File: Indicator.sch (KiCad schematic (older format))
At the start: 6 parts, among them U10 BC56-12SURKWA, U11 SC56-11SRWA, U12 MAX7219EWG+T, U8 CC56-12SURKWA, U9 MAX7219EWG+T

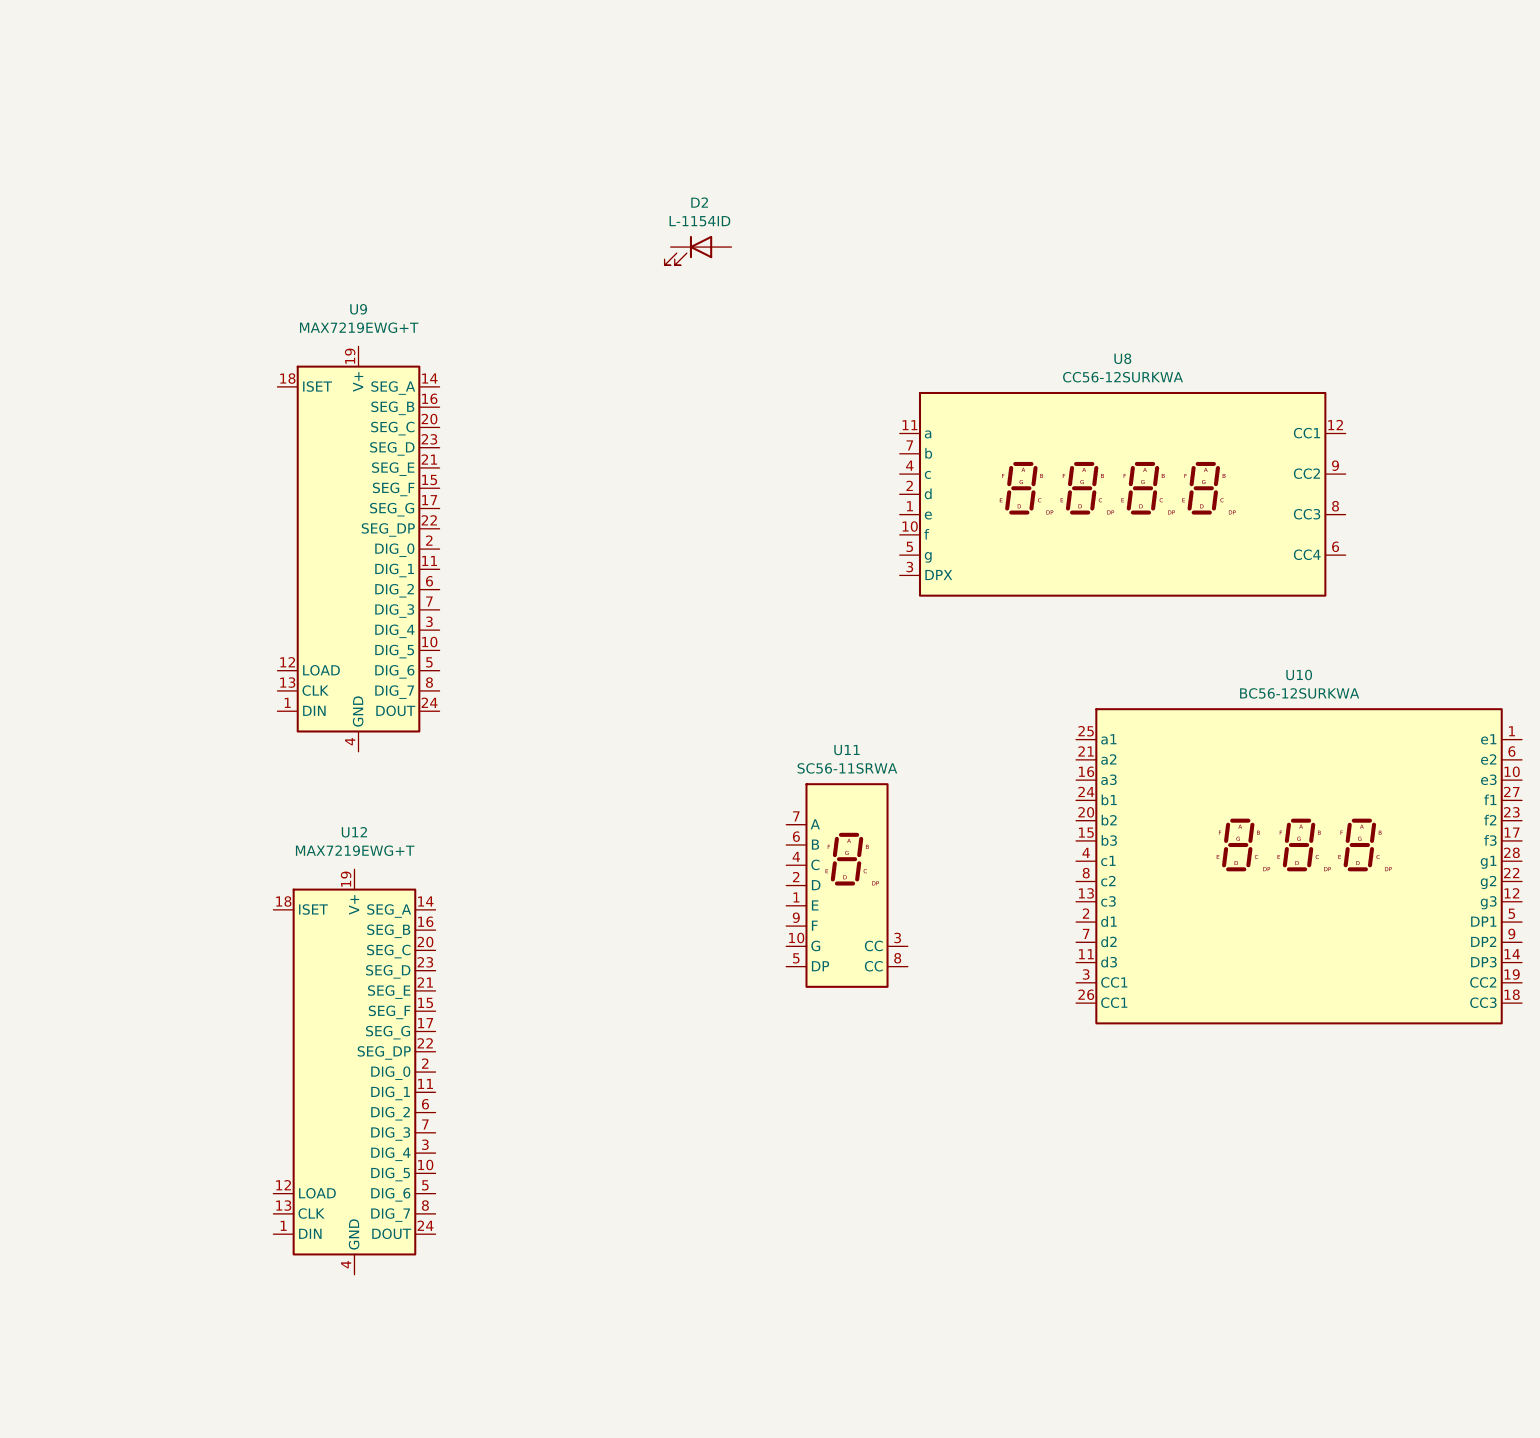
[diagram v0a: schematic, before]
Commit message: Indication edit
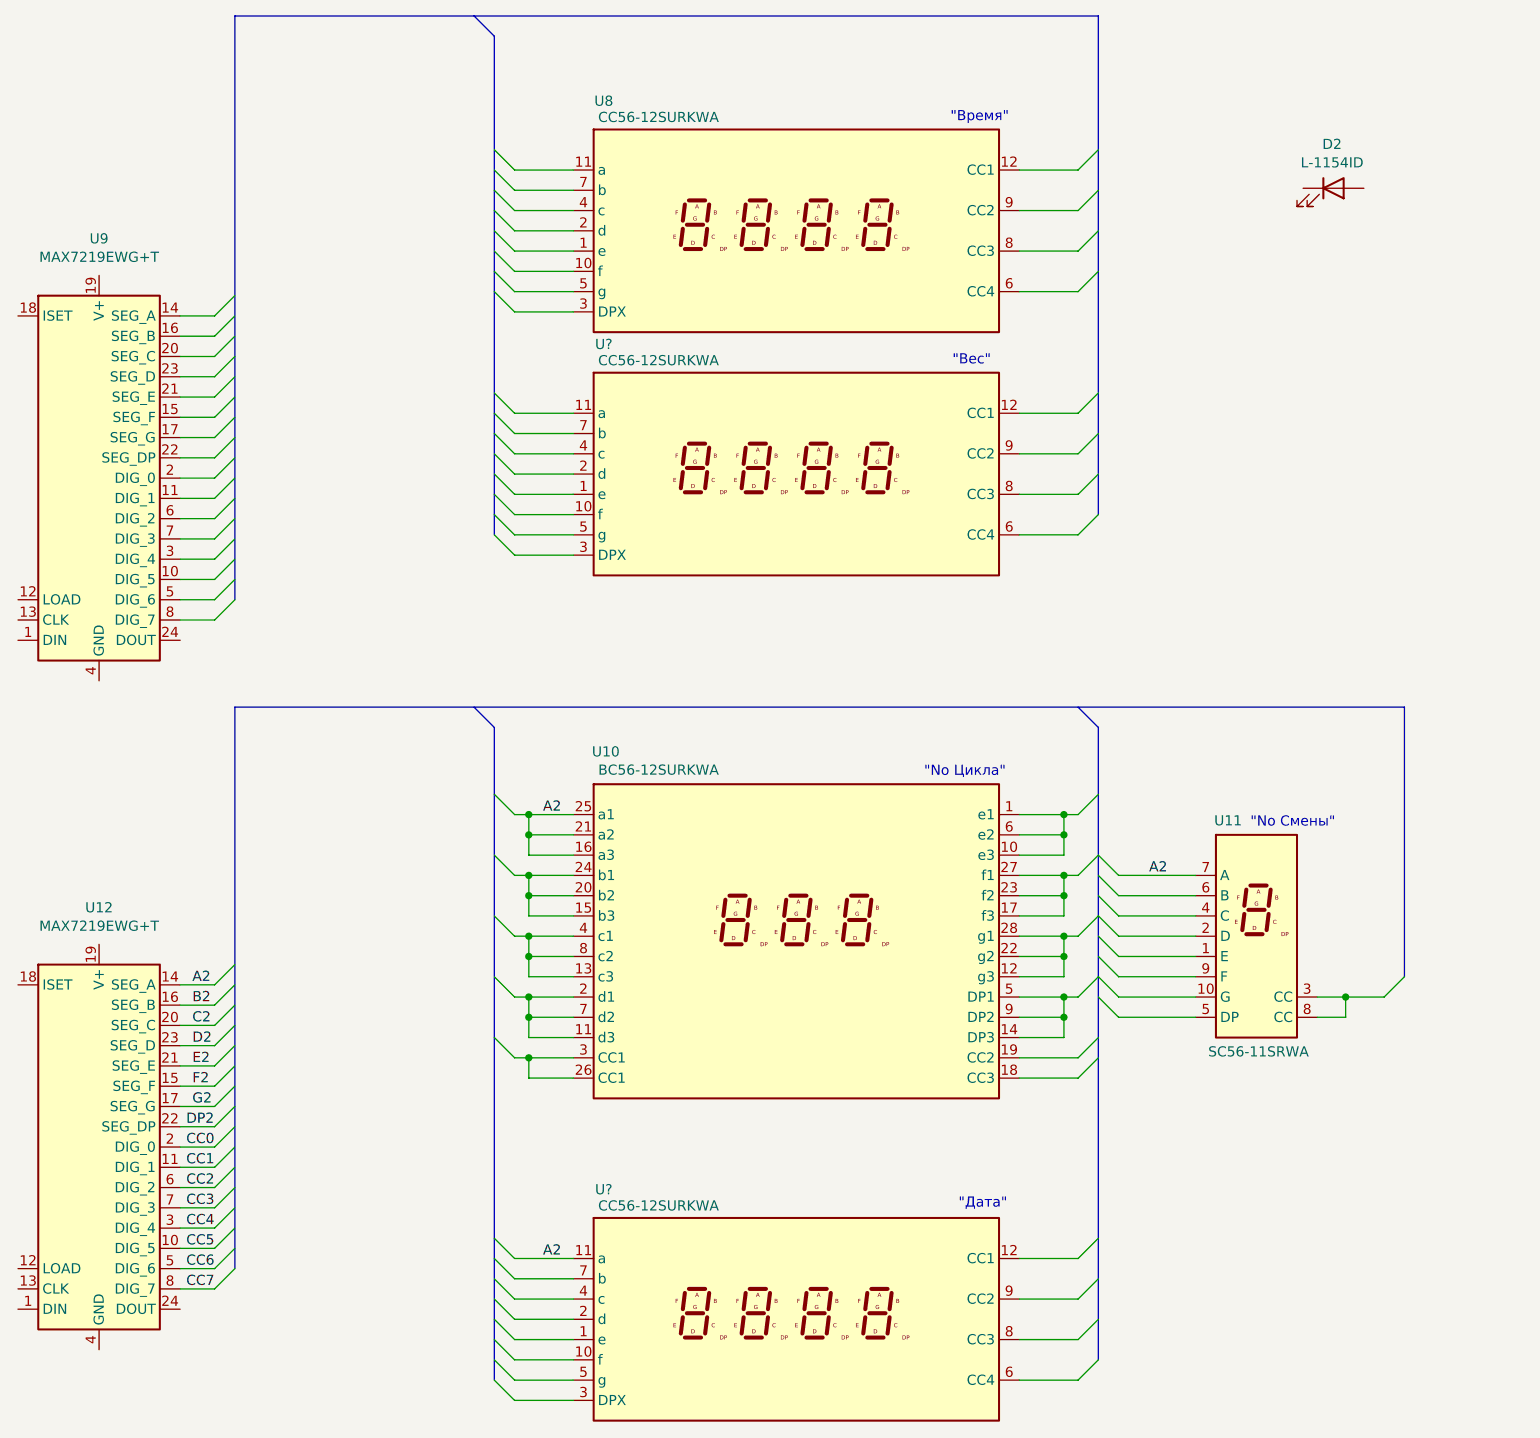
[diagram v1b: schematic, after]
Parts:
- added U? (x2): CC56-12SURKWA, Display_7Segment:CA56-12SURKWA, symbol SVIELCOM_Library:CC56-12SURKWA
- U10: footprint Display_7Segment:CA56-12SURKWA -> SVIELCOM:BC56-11SURKWA
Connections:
- net CC5: now reaches U12.10 (DIG_5)
- net CC1: now reaches U12.11 (DIG_1)
- net A2: now reaches U12.14 (SEG_A)
- net A2: now also U10.16 (a3), U10.21 (a2), U10.25 (a1), U11.7 (A), U?.11 (a)
- net F2: now reaches U12.15 (SEG_F)
- net B2: now reaches U12.16 (SEG_B)
- net G2: now reaches U12.17 (SEG_G)
- net CC0: now reaches U12.2 (DIG_0)
- net C2: now reaches U12.20 (SEG_C)
- net E2: now reaches U12.21 (SEG_E)
- net DP2: now reaches U12.22 (SEG_DP)
- net D2: now reaches U12.23 (SEG_D)
- net CC4: now reaches U12.3 (DIG_4)
- net CC6: now reaches U12.5 (DIG_6)
- net CC2: now reaches U12.6 (DIG_2)
- net CC3: now reaches U12.7 (DIG_3)
- net CC7: now reaches U12.8 (DIG_7)
- net at U11.3 (CC): now also U11.8 (CC)
- net at U10.1 (e1): now also U10.10 (e3), U10.6 (e2)
- net at U10.11 (d3): now also U10.2 (d1), U10.7 (d2)
- net at U10.12 (g3): now also U10.22 (g2), U10.28 (g1)
- net at U10.13 (c3): now also U10.4 (c1), U10.8 (c2)
- net at U10.14 (DP3): now also U10.5 (DP1), U10.9 (DP2)
- net at U10.15 (b3): now also U10.20 (b2), U10.24 (b1)
- net at U10.17 (f3): now also U10.23 (f2), U10.27 (f1)
- net at U10.26 (CC1): now also U10.3 (CC1)
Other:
- note added: ""No Смены""
- note added: ""No Цикла""
- note added: ""Вес""
- note added: ""Время""
- note added: ""Дата""
- moved on the sheet: D2, U10, U11, U12, U8, U9
